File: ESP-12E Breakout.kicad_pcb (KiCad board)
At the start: 2 copper layers, 40 x 40 mm, 6 parts, among them J3 Conn_01x08_Pin, J4 Conn_01x08_Pin, J5 Conn_01x06_Pin, U1 ESP-12E

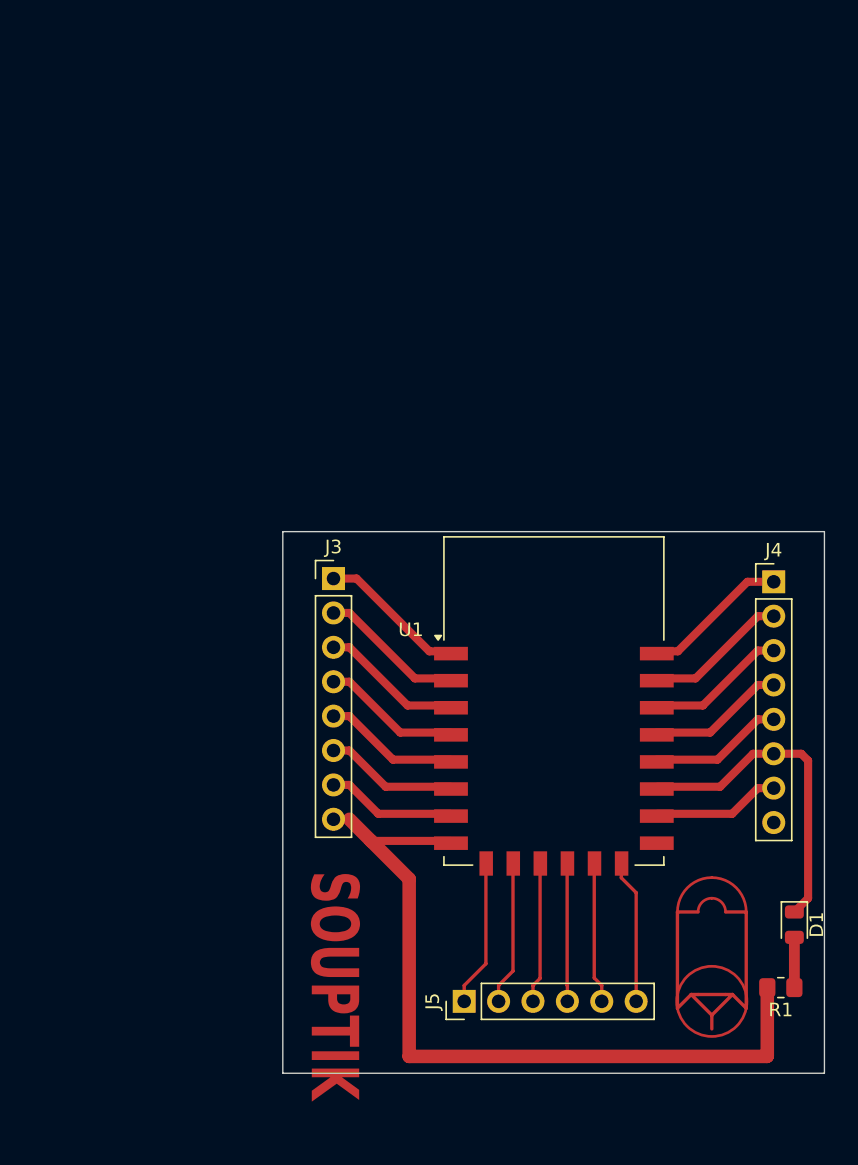
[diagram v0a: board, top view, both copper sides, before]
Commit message: Add files via upload
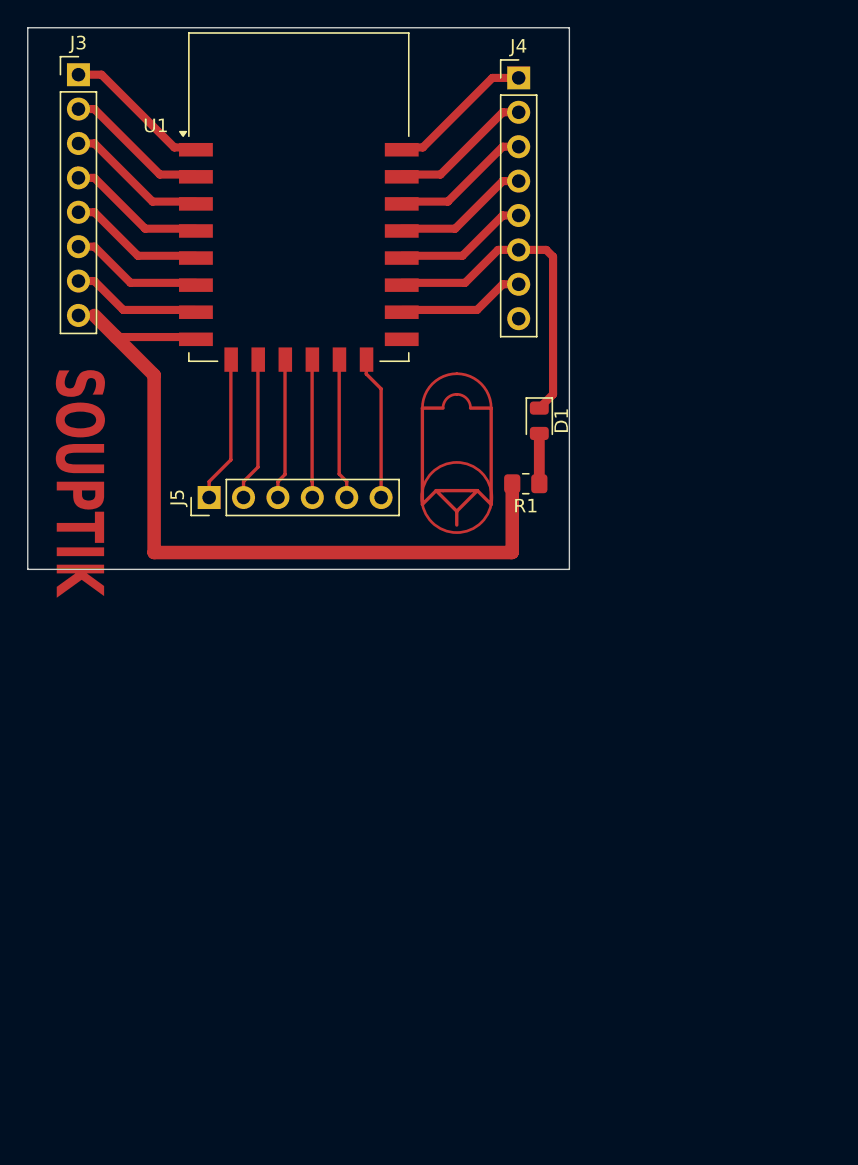
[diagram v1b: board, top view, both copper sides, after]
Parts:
- moved D1 41.7 mm to (131.0, 76.5)
- moved J3 41.7 mm to (97.0, 50.9)
- moved R1 41.7 mm to (130.0, 81.2)
- moved J4 41.7 mm to (129.5, 51.2)
- moved U1 41.7 mm to (113.3, 60.0)
- moved J5 41.7 mm to (106.6, 82.2)
